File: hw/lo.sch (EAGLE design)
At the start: 45 parts, among them U1 ADF4360-9, X1 CLK, X2 DATA, X3 LE, X4 DIVOUT, X5 SMA-142-0701-881/886, X6 SMA-142-0701-881/886, X7 VIN

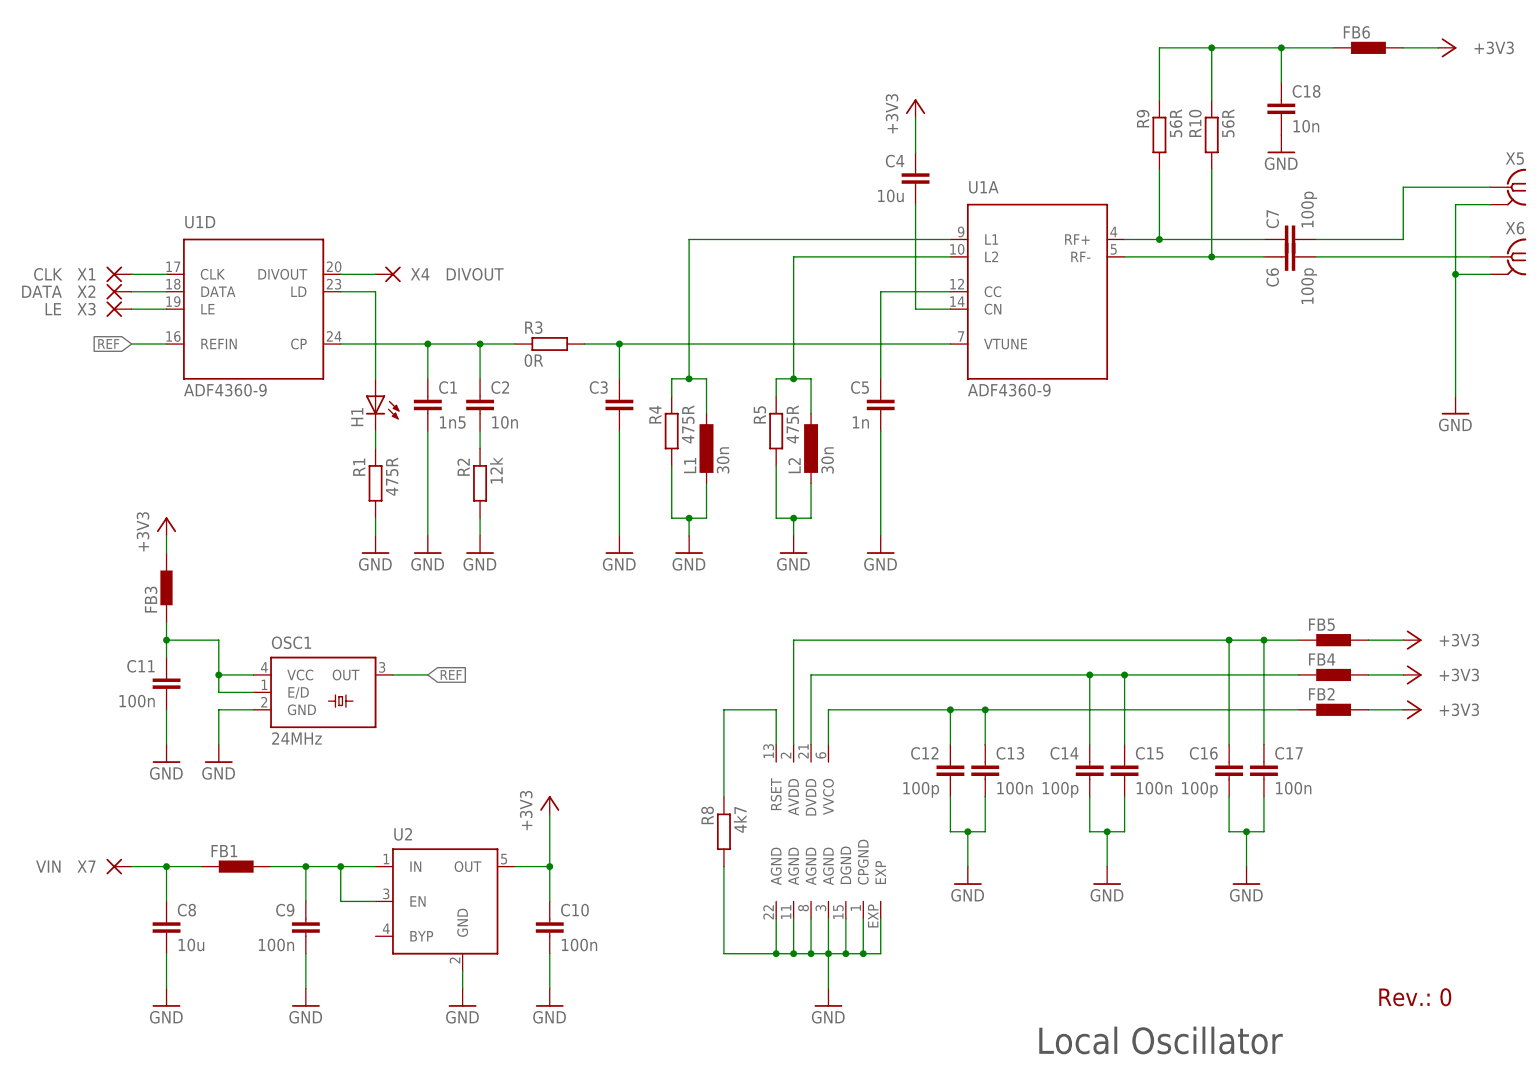
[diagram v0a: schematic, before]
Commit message: rev.1: finished lo board
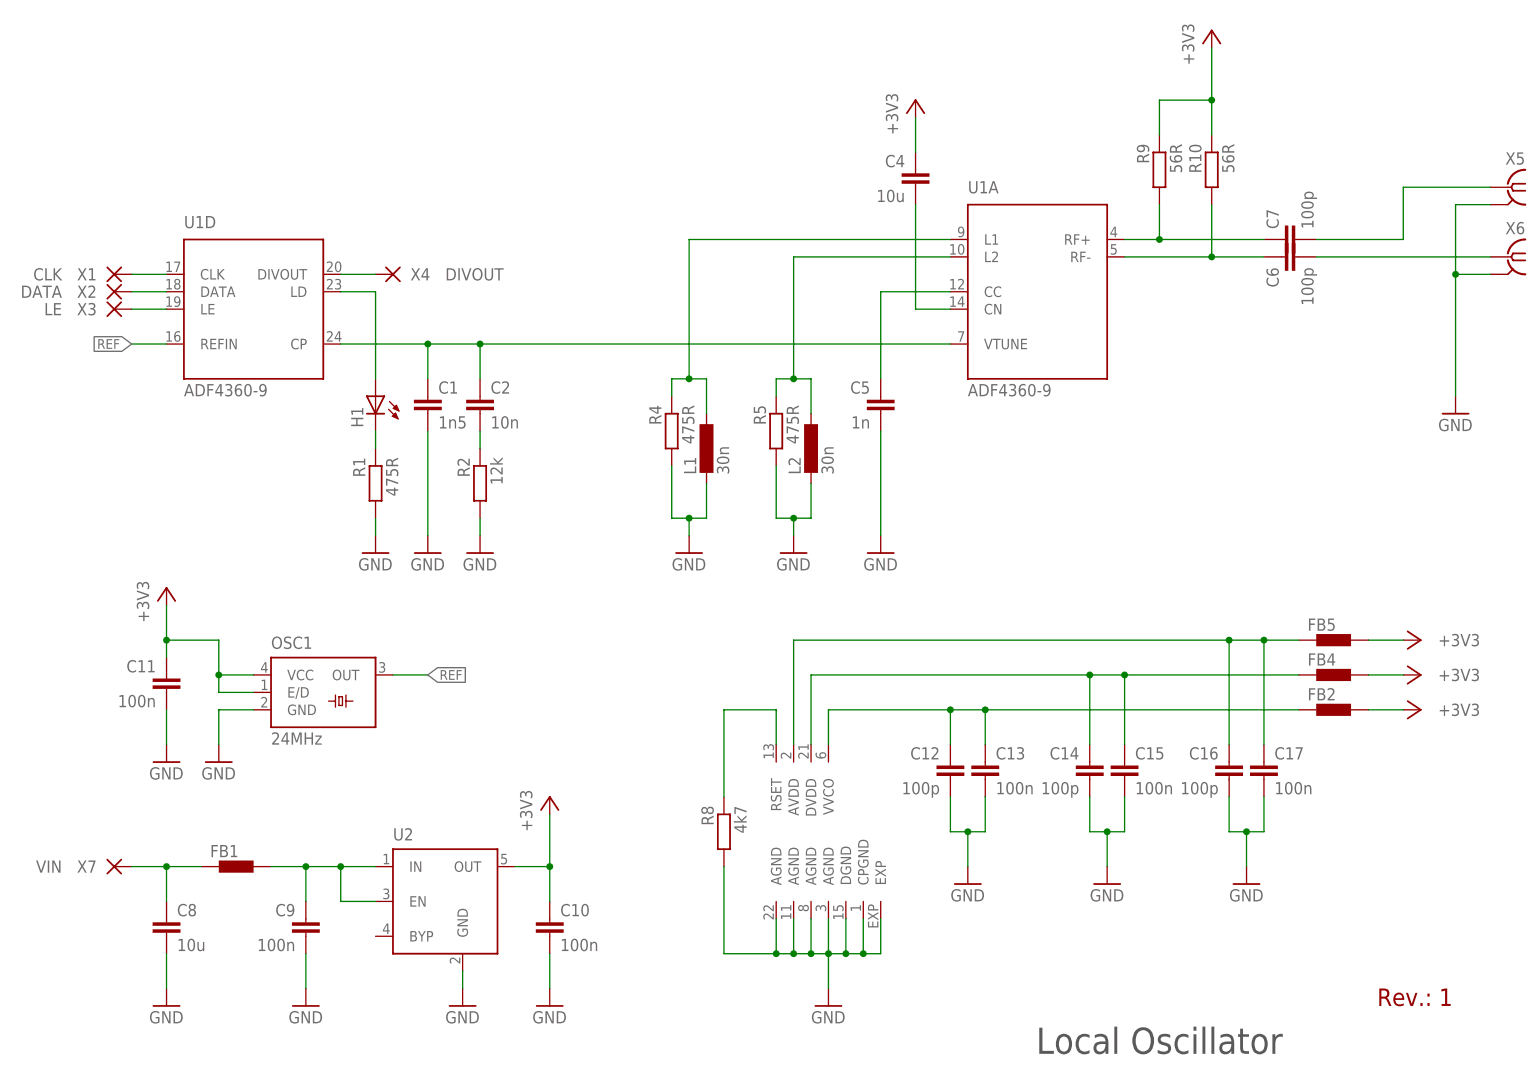
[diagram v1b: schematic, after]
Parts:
- removed C18: 10n, rcl:C-EUC0402
- removed C3: (no value), rcl:C-EUC0402
- removed FB3, FB6: BML15H, ferrite-bead:BML15H
- removed R3: 0R, rcl:R-EU_R0603
- L1, L2: device rcl:L-EUL4532C -> rcl:L-EUL2012C
- R8: device rcl:R-EU_R0603 -> rcl:R-EU_R0402
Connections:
- net N$11 renamed RUT
- removed net N$10: C3.1, R3.2, U1A.VTUNE
- removed net N$21: C18.1, FB6.1, R10.1, R9.1
- removed net N$27: C11.1, FB3.1, OSC1.E/D, OSC1.VCC
- removed net N$7: C1.1, C2.1, R3.1, U1D.CP
- new net LD: C1.1, C2.1, U1A.VTUNE, U1D.CP
- net +3V3: now also C11.1, OSC1.E/D, OSC1.VCC, R10.1, R9.1; no longer FB3.2, FB6.2
- net GND: no longer C18.2, C3.2
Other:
- note added: "Rev.: 1"
- note removed: "Rev.: 0"
- moved on the sheet: R10, R9
